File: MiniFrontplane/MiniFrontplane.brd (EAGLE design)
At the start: 95.7 x 39.4 mm, 17 parts, among them IC2 74ACT14N, U1 MCP130SOT

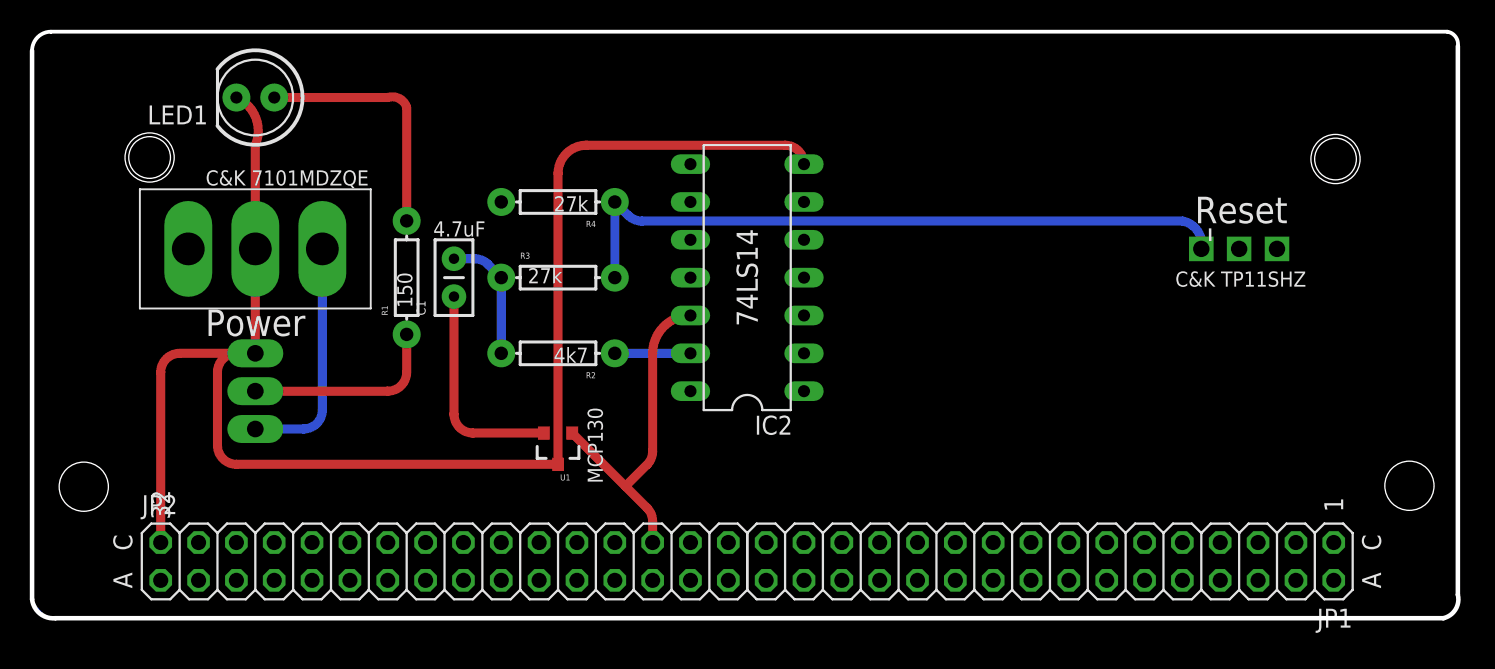
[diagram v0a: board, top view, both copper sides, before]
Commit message: Frontplane THAT MIGHT WORK THIS TIME
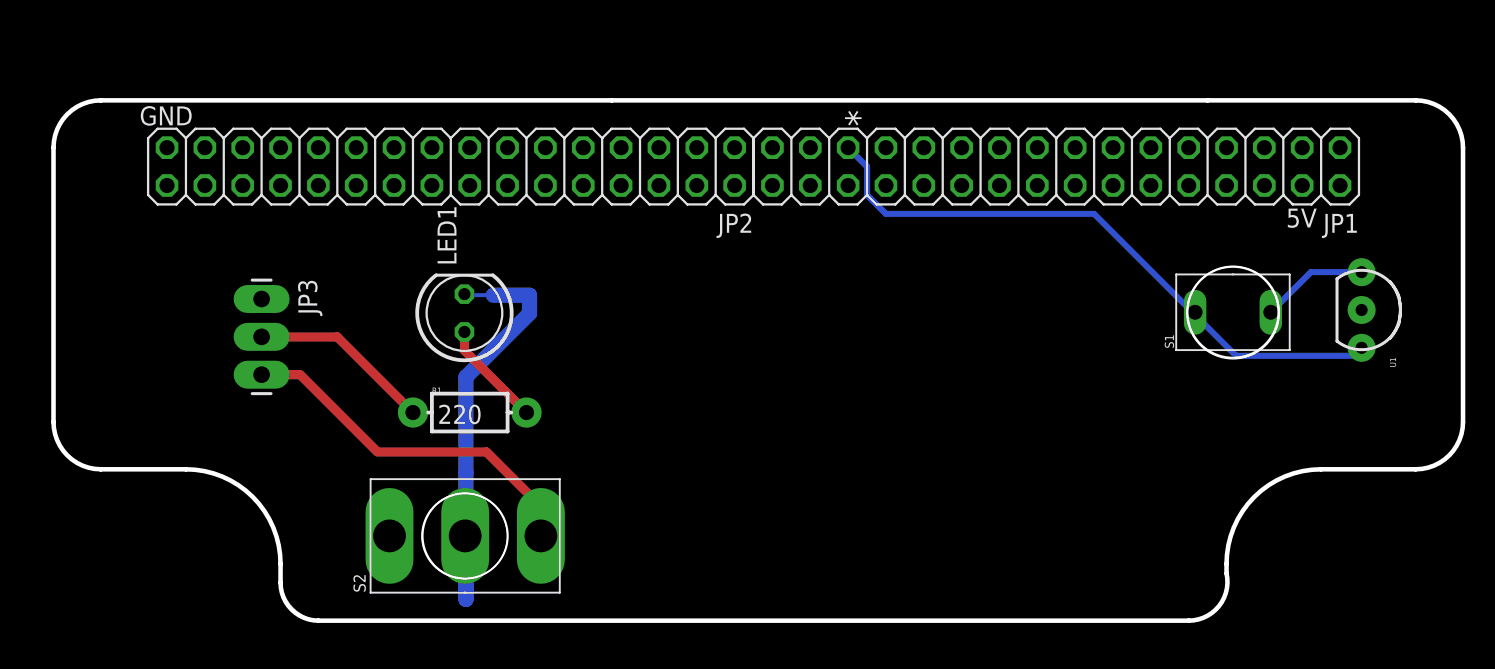
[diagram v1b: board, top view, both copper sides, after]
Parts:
- removed C1: 4.7uF, SparkFun-Passives:CAP-PTH-SMALLEZ
- removed IC2: 74ACT14N, 74xx-eu:DIL14
- removed R2: 4k7, SparkFun-Resistors:AXIAL-0.3
- removed R3, R4: 27k, SparkFun-Resistors:AXIAL-0.3
- removed U$1: MINITOGGLE, Benchoff:MINITOGGLE
- removed U$2: MINITACT, Benchoff:MINITACT
- removed U$22, U$4, U$5, U$9: (no value), SparkFun-Electromechanical:STAND-OFF
- added S1: TP11SWITCH, Benchoff:TP11
- added S2: MINITOGGLE, Benchoff:MINITOGGLE
- JP3: value Samtec SLW-103-01-T-S -> (none)
- LED1: device SparkFun-LED:LED5MM -> led:LED5MM
- R1: value 150 -> 220; device SparkFun-Resistors:AXIAL-0.3 -> SparkFun-Resistors:AXIAL-0.3-KIT
- U1: value MCP130SOT -> DS1813; device SparkFun-DigitalIC:SOT23-3 -> Benchoff:TO-92
- moved U1 54.7 mm to (91.6, 22.1), turned to 270 degrees
- moved JP1 26.5 mm to (71.1, 31.8)
- moved JP2 26.5 mm to (30.5, 31.8), turned to 180 degrees
- moved LED1 20.2 mm to (31.4, 21.9), turned to 90 degrees
- moved R1 10.00 mm to (31.8, 15.2), turned to 0 degrees
- moved JP3 8.74 mm to (17.8, 22.9), flipped to the top, turned to 270 degrees
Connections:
- net N$2 renamed PS_OK
- removed net 5VSB: JP1.3
- removed net N$1 (its old number): JP3.1, U$1.P2
- removed net N$4: R3.P$2, R4.P$1, U$2.CON2
- removed net N$5: C1.2, R2.P$2, R3.P$1
- removed net N$6: IC2.13, R2.P$1
- new net PS_ON: JP3.3, S2.L2
- net GND: now also JP2.31, JP3.1, S1.P$2, S2.COM; no longer IC2.7, JP2.2, JP3.3, R4.P$2, U$1.COM
- net RESET: now also JP1.27, S1.P$1; no longer IC2.12, JP2.28
- net VCC: no longer C1.1, IC2.14, U$2.CON1
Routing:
- net GND: track 104.4 -> 38.1 mm
- net N$4: track 45.9 -> 0.00 mm
- net PS_ON: track 0.00 -> 24.4 mm
- net RESET: track 22.7 -> 41.7 mm
- net N$1 (its old number): track 15.8 -> 0.00 mm
- net VCC: track 14.5 -> 0.00 mm
- net N$1: track 16.7 -> 7.14 mm
- net N$5: track 8.70 -> 0.00 mm
- net N$6: track 5.08 -> 0.00 mm
- net PS_OK: track 13.2 -> 12.3 mm
- added copper zone on layer 16, net GND
- added copper zone on layer 1, net VCC
- removed copper zone on layer 1, net GND
- removed copper zone on layer 16, net VCC
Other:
- board size 95.7 x 39.4 mm -> 94.6 x 34.9 mm
- board text added: "*"
- board text added: "5V"
- board text added: "64 Pin Terminal Samtek TLW-132-06-F-D SLW-132-01-F-D"
- board text added: "GND"
- board text removed: "1"
- board text removed: "32"
- board text removed: "4.7uF"
- board text removed: "74LS14"
- board text removed: "A"
- board text removed: "C"
- board text removed: "C&K 7101MDZQE"
- board text removed: "C&K TP11SHZ"
- board text removed: "MCP130"
- board text removed: "Power"
- board text removed: "Reset"
